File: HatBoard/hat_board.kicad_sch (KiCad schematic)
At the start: 19 parts, among them J1 DF11 FC Connection, J13 DF11 FC Connection, J2 Conn_01x04, J20 DF11 FC Connection, J21 DF11 FC Connection, U10 VEML7700, U12 DRV2605LDGS, U27 TMP112AIDRLR

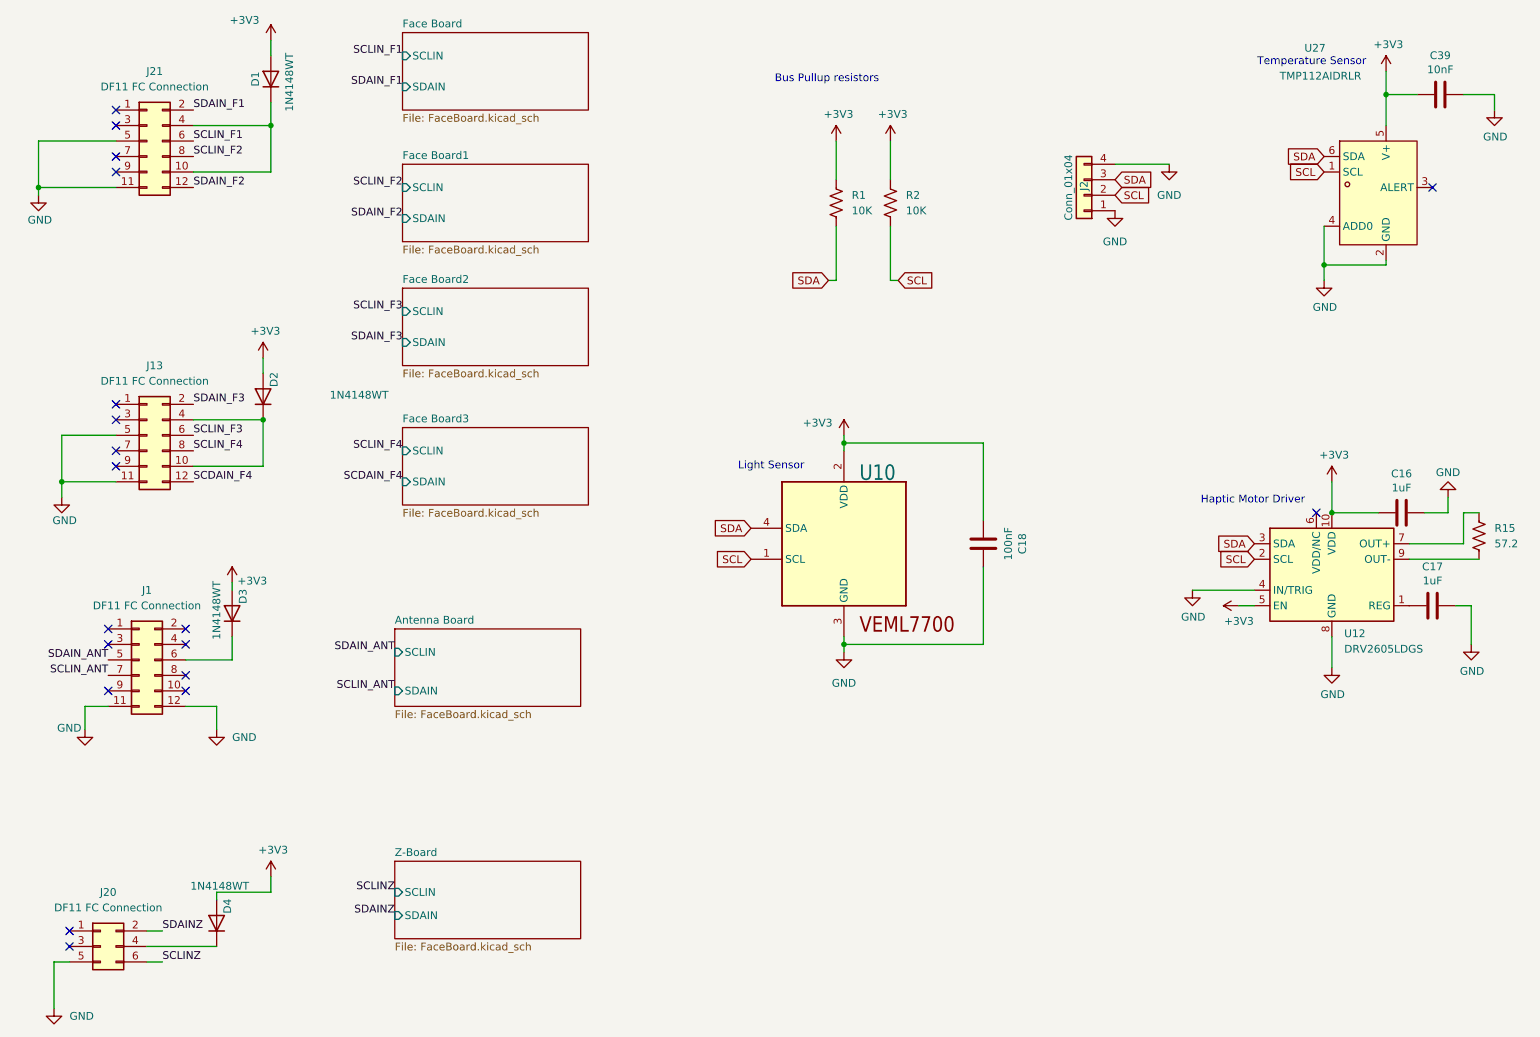
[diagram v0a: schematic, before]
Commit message: diode added
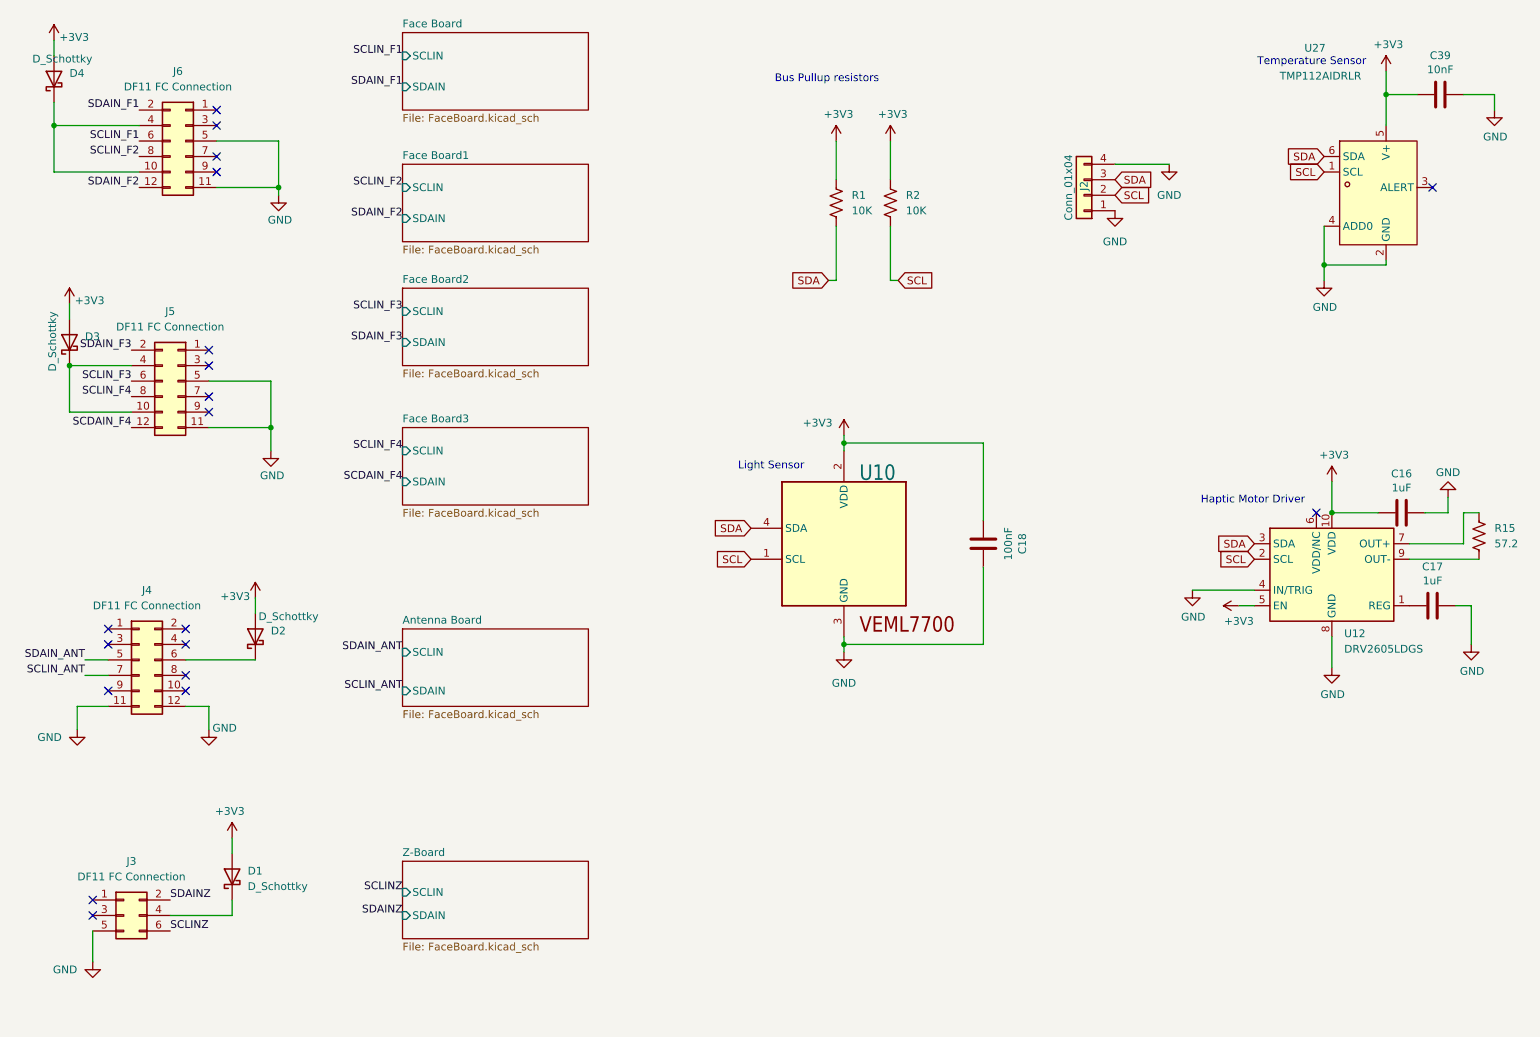
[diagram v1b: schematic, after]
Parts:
- removed D1, D2, D3, D4: 1N4148WT, Diode_SMD:D_SOD-523, symbol Diode:1N4148WT
- removed J1, J13, J21: DF11 FC Connection, easyeda2kicad:CONN-TH_DF11-12DS-2DSA-05, symbol Connector_Generic:Conn_02x06_Odd_Even
- removed J20: DF11 FC Connection, easyeda2kicad:CONN-TH_DF11-12DS-2DSA-05, symbol Connector_Generic:Conn_02x03_Odd_Even
- added D1, D2, D3, D4: D_Schottky, easyeda2kicad:POWERDI-123_L2.8-W1.8-LS3.7-RD, symbol Device:D_Schottky
- added J3: DF11 FC Connection, easyeda2kicad:CONN-TH_DF11-12DS-2DSA-05, symbol Connector_Generic:Conn_02x03_Odd_Even
- added J4, J5, J6: DF11 FC Connection, easyeda2kicad:CONN-TH_DF11-12DS-2DSA-05, symbol Connector_Generic:Conn_02x06_Odd_Even
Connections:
- net +3V3: now also D1.2 (A), D2.2 (A), D3.2 (A), D4.2 (A)
- net GND: now also J3.5 (Pin_5), J4.11 (Pin_11), J4.12 (Pin_12), J5.11 (Pin_11), J5.5 (Pin_5), J6.11 (Pin_11), J6.5 (Pin_5)
- net SCDAIN_F4: now also J5.12 (Pin_12)
- net SCLINZ: now also J3.6 (Pin_6)
- net SCLIN_ANT: now also J4.7 (Pin_7)
- net SCLIN_F1: now also J6.6 (Pin_6)
- net SCLIN_F2: now also J6.8 (Pin_8)
- net SCLIN_F3: now also J5.6 (Pin_6)
- net SCLIN_F4: now also J5.8 (Pin_8)
- net SDAINZ: now also J3.2 (Pin_2)
- net SDAIN_ANT: now also J4.5 (Pin_5)
- net SDAIN_F1: now also J6.2 (Pin_2)
- net SDAIN_F2: now also J6.12 (Pin_12)
- net SDAIN_F3: now also J5.2 (Pin_2)
- new net: D2.1 (K), J4.6 (Pin_6)
- new net: D4.1 (K), J6.10 (Pin_10), J6.4 (Pin_4)
- new net: D1.1 (K), J3.4 (Pin_4)
- new net: D3.1 (K), J5.10 (Pin_10), J5.4 (Pin_4)

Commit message: Changed Footprint of 56R
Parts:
- R15: footprint Resistor_SMD:R_0201_0603Metric_Pad0.64x0.40mm_HandSolder -> Resistor_SMD:R_0603_1608Metric
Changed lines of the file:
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@@
 			)
 		)
-		(property "Footprint" "Resistor_SMD:R_0201_0603Metric_Pad0.64x0.40mm_HandSolder"
+		(property "Footprint" "Resistor_SMD:R_0603_1608Metric"
 			(at 253.746 108.204 90)
 			(effects
